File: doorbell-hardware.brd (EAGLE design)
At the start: 100 x 80 mm, 11 parts, among them IC1 REG1117, T1 BC846

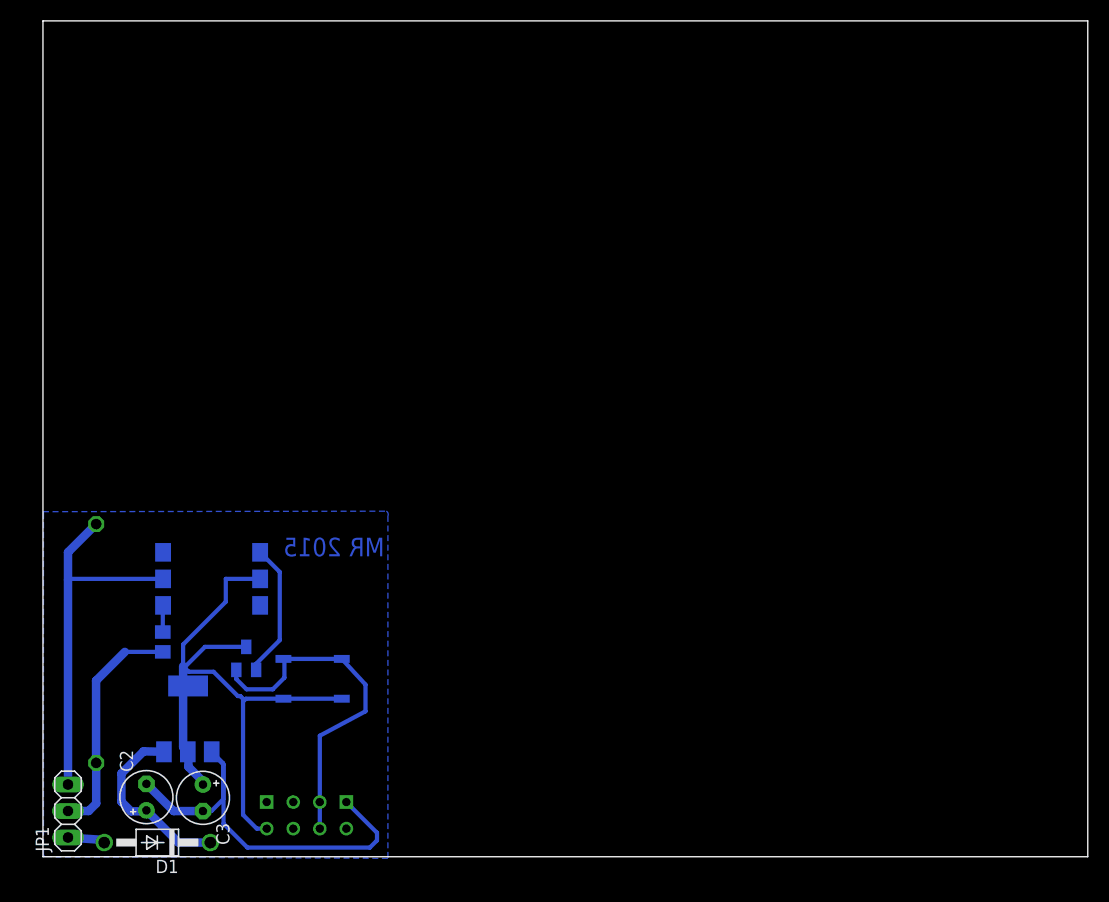
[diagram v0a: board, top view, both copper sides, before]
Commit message: Working schematic and smaller layout
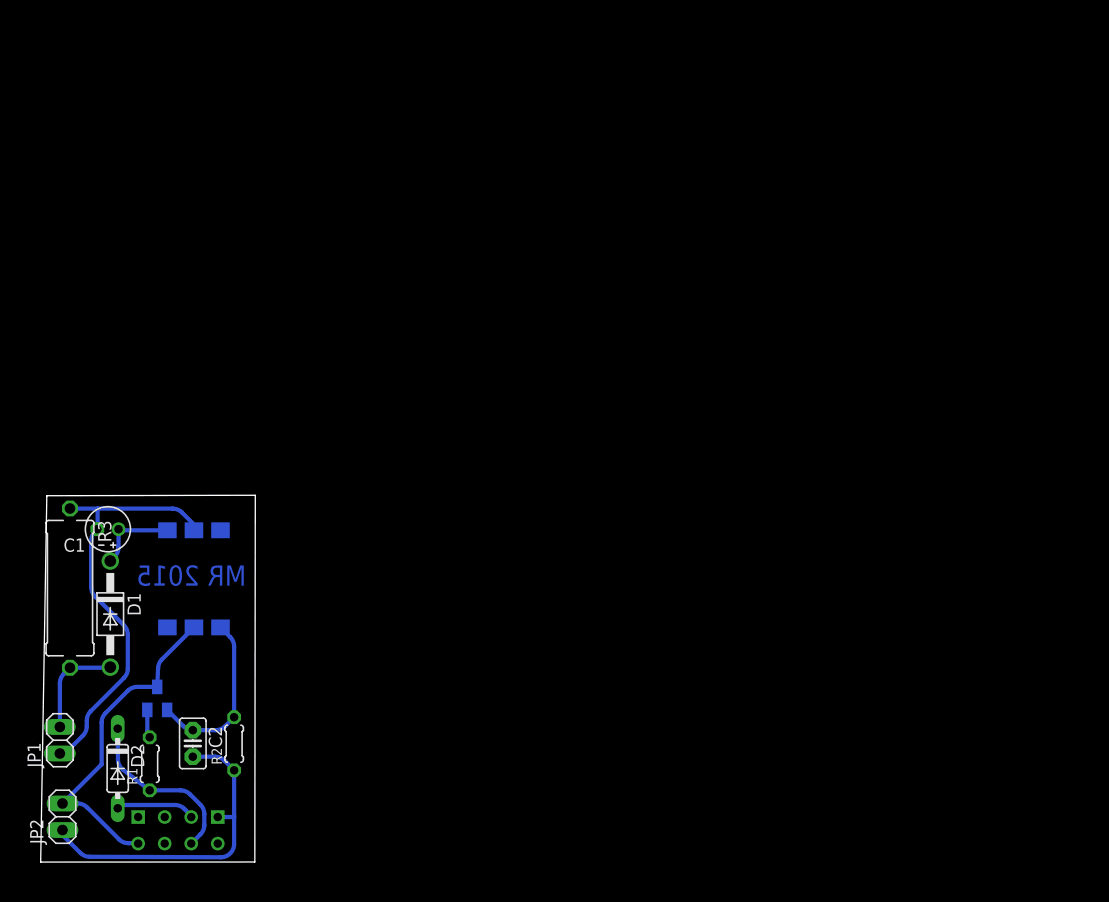
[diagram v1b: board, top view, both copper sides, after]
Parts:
- removed C3: 100u, rcl:E2,5-5
- removed IC1: REG1117, burr-brown:SOT223
- removed S1: TAC_SWITCHSMD, SparkFun-Electromechanical:TACTILE-SWITCH-SMD
- added C1: 220u, resistor:E2-4
- added D2: 1N4148DO35-7, diode:DO35-7
- added JP2: (no value), pinhead:1X02
- added R2: 1.2k, resistor:0204/5
- C2: value 10u -> 0.1u; device rcl:E2,5-5 -> capacitor-wima:C2.5-2
- D1: value 1N4004 -> BAT49
- JP1: device pinhead:1X03 -> pinhead:1X02
- R1: value 2.4 -> 56k; device resistor:0922/22 -> resistor:0204/5
- R3: value 1k -> 2.4; device eagle-ltspice:R0805 -> resistor:P0613/15
- moved D1 22.3 mm to (6.44, 23.2), turned to 270 degrees
- moved R1 12.6 mm to (10.2, 8.89), flipped to the top, turned to 90 degrees
- moved U$1 12.4 mm to (12.9, 9.44)
- moved R3 10.3 mm to (2.59, 25.7), flipped to the top
- moved T1 9.34 mm to (10.9, 15.2)
- moved JP1 6.82 mm to (1.62, 11.2)
- moved C2 6.79 mm to (14.3, 10.8), turned to 270 degrees
- moved OK1 1.69 mm to (14.5, 26.6), turned to 180 degrees
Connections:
- removed net AC+: D1.A, JP1.1
- removed net AC-: JP1.2, R1.2, R3.2
- new net N$6: C2.1, OK1.4, R2.2, T1.1
- new net N$9: D2.A, U$1.GPIO2
- net BUTTON: now also D2.C, R1.1; no longer S1.1, S1.2, T1.2, U$1.GPIO2
- net GND: now also C2.2, JP2.1, R2.1; no longer C2.-, C3.-, IC1.1
- net N$1: now also D1.A, JP1.2, R3.2; no longer C2.+, D1.C, IC1.3
- net N$2: now also R1.2, T1.2; no longer JP1.3, OK1.2, R1.1
- net N$3: now also C1.+, D1.C; no longer R3.1
- net N$4: now also C1.-, JP1.1, OK1.2, R3.1; no longer OK1.4, T1.1
- net VCC: now also JP2.2; no longer C3.+, IC1.2, S1.3, S1.4
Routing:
- net N$2: track 35.2 -> 2.67 mm
- net VCC: track 62.7 -> 31.9 mm
- net N$4: track 13.0 -> 40.5 mm
- net AC-: track 22.8 -> 0.00 mm
- net BUTTON: track 33.5 -> 16.9 mm
- net N$6: track 0.00 -> 16.6 mm
- net GND: track 42.0 -> 31.2 mm
- net N$1: track 17.9 -> 9.87 mm
- net N$9: track 0.00 -> 7.64 mm
- net N$3: track 2.56 -> 7.99 mm
- net AC+: track 3.84 -> 0.00 mm
- removed copper zone on layer 16, net N$5
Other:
- board size 100 x 80 mm -> 20.5 x 35.1 mm
